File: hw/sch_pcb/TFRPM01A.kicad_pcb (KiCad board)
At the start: 2 copper layers, 37.5 x 19.1 mm, 25 parts, among them J1 HEADER_1x03, J2 SM04B-GHS-TB, J3 SM04B-GHS-TB, U1 PCF8583, U2 74AHC1G14GV, U3 MIC5504-3.3YM5

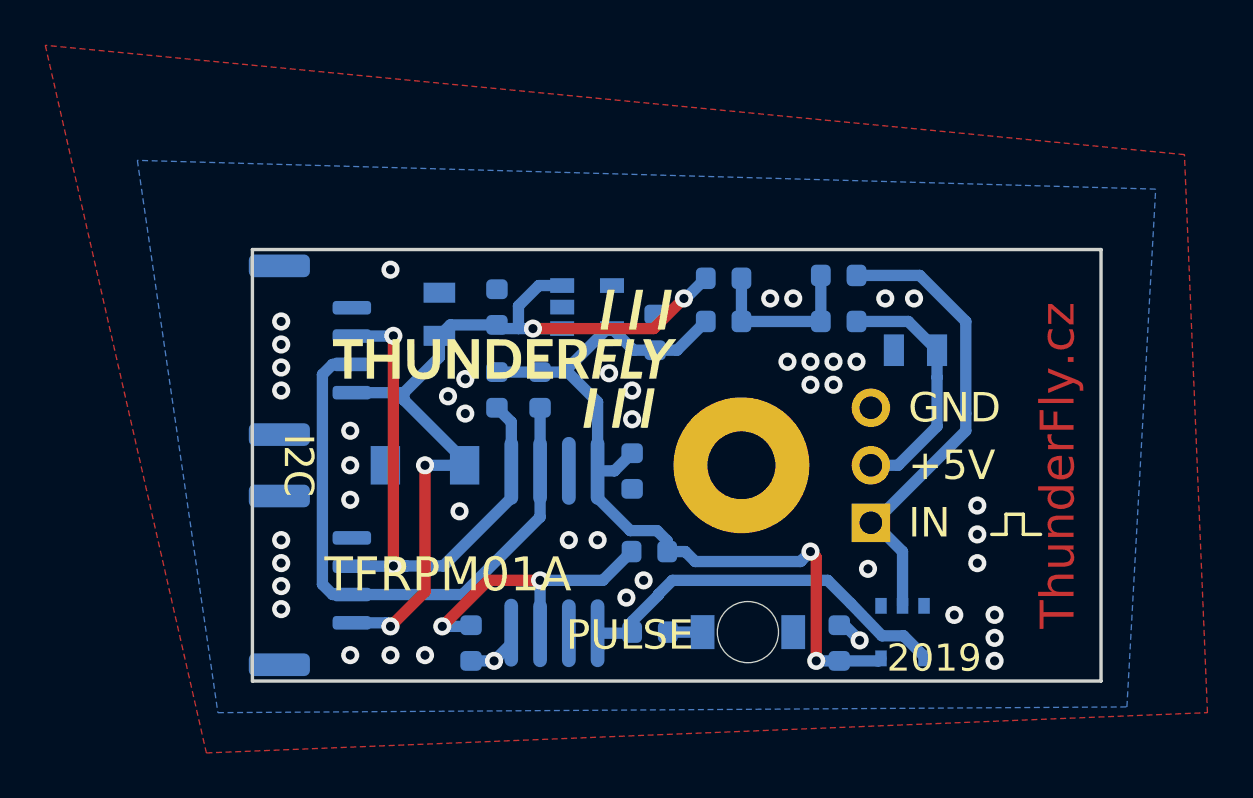
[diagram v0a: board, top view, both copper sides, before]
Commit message: Edit
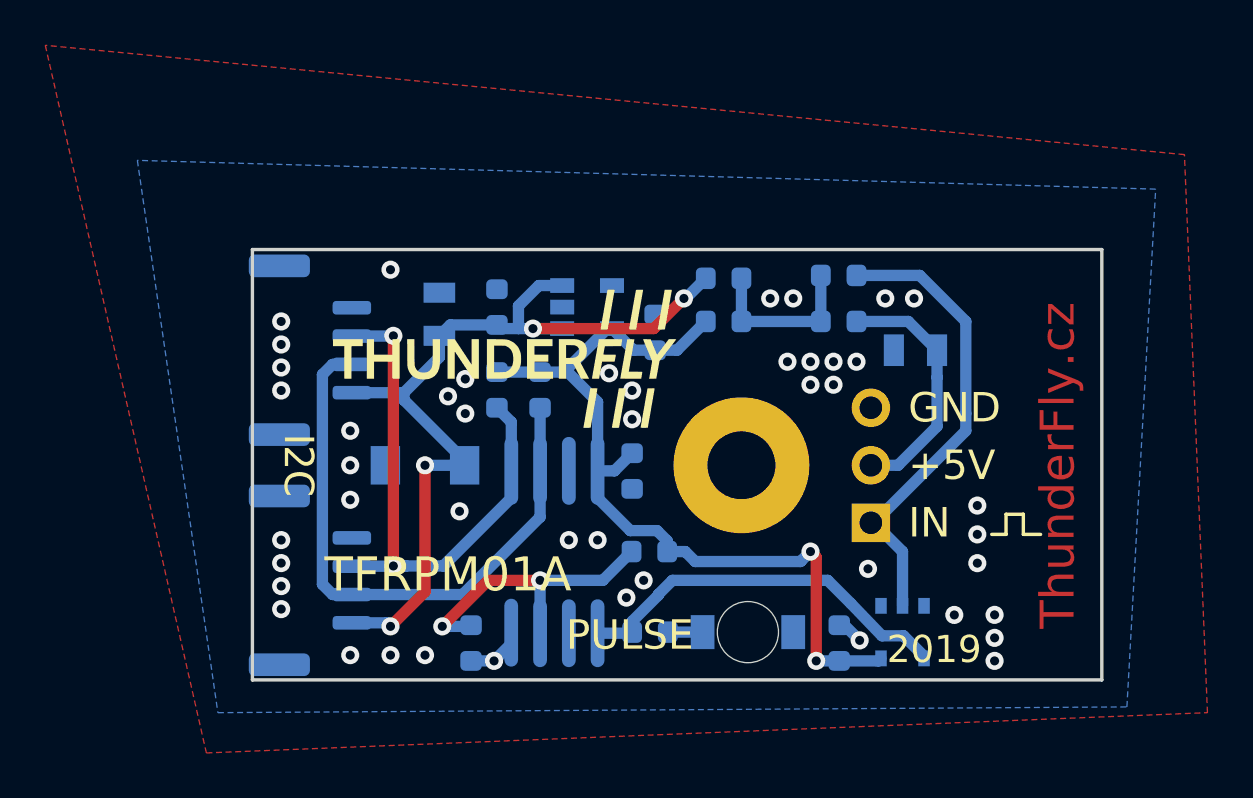
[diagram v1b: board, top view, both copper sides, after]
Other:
- board size 37.5 x 19.1 mm -> 37.5 x 19 mm
